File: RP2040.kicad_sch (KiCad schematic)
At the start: 28 parts, among them J3 USB_C_Receptacle_USB2.0_16P, U1 RP2040, U2 AMS1117-3.3, U4 W25Q16JVSS, Y1 X322512MSB4SI

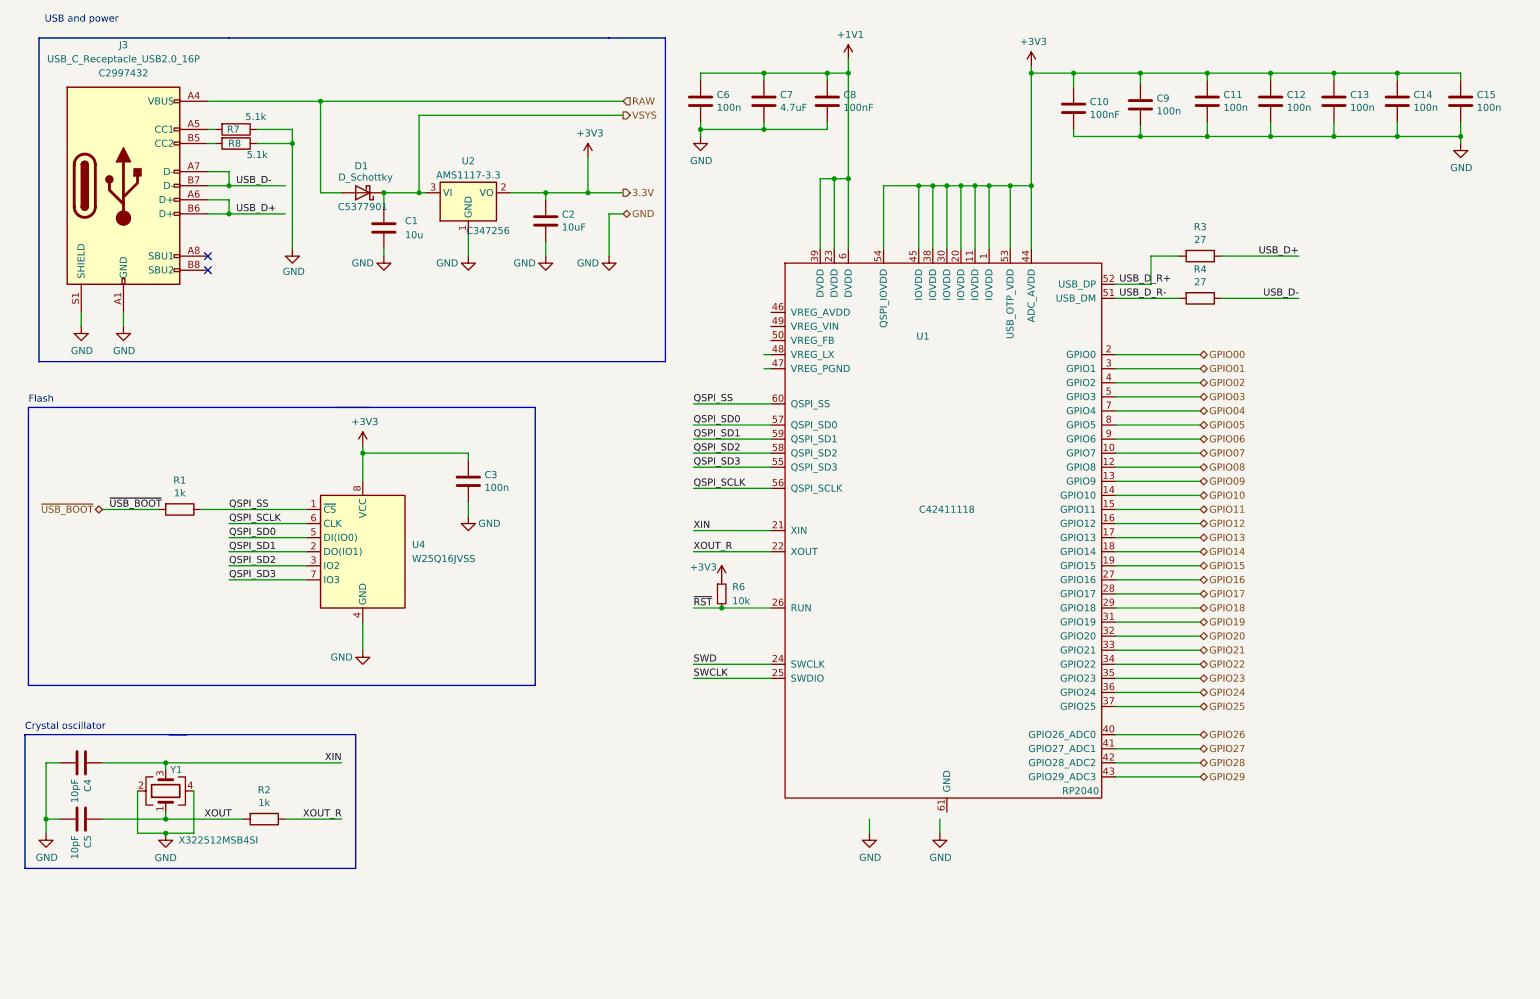
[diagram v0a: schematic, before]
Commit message: fixed all warnings/errors
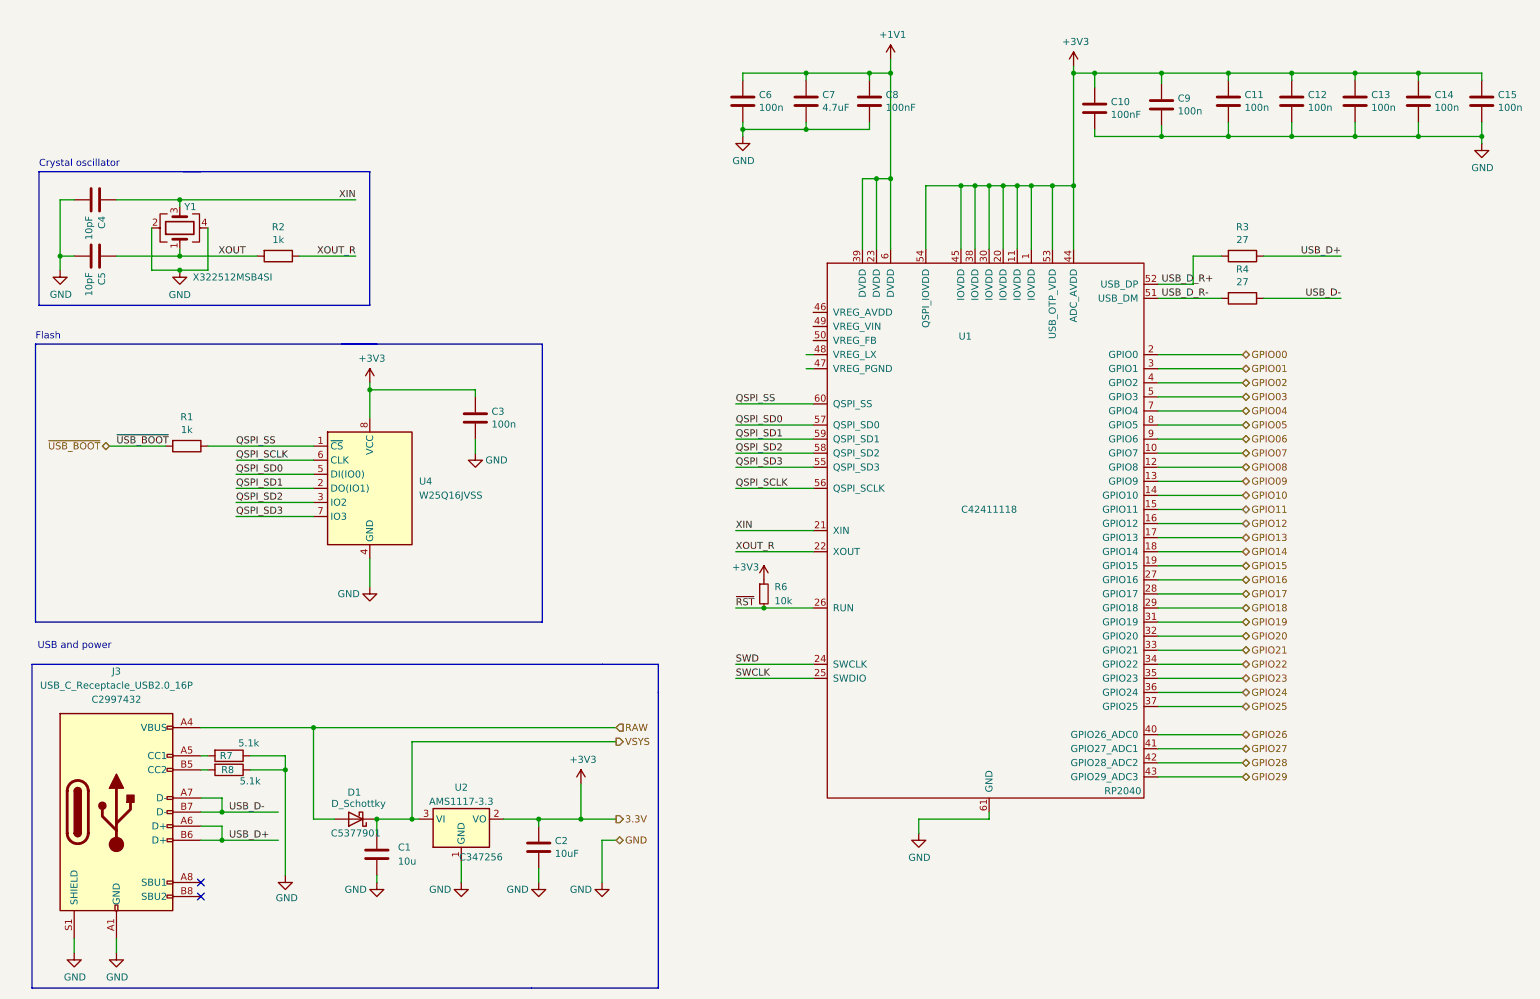
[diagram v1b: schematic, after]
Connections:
- net GND: now also U1.61 (GND)
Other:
- moved on the sheet: C1, C10, C11, C12, C13, C14, C15, C2, C3, C4, C5, C6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
